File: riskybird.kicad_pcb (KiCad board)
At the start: 2 copper layers, 58.3 x 58.3 mm, 81 parts, among them J1 USB_B_Micro, J2 Conn_01x02, J3 Conn_01x02, J4 Conn_01x02, J5 Conn_01x02, J6 Conn_01x02, J7 Conn_01x10, J8 Conn_01x10, Q1 SI2302, Q2 SI2302, Q3 SI2302, Q4 SI2302, Q5 DNBT8105-7, Q6 DNBT8105-7, Q7 Q_NMOS_GSD, SW1 SW_SPST, SW2 SW_SPST, SW3 SW_SPST, U1 MCP73831-2-OT, U10 74LVC2G08, U3 TPS2113A, U4 LP2985-3.0, U6 ESP32-C3-WROOM-02, U7 BMI088, U8 FT231XS

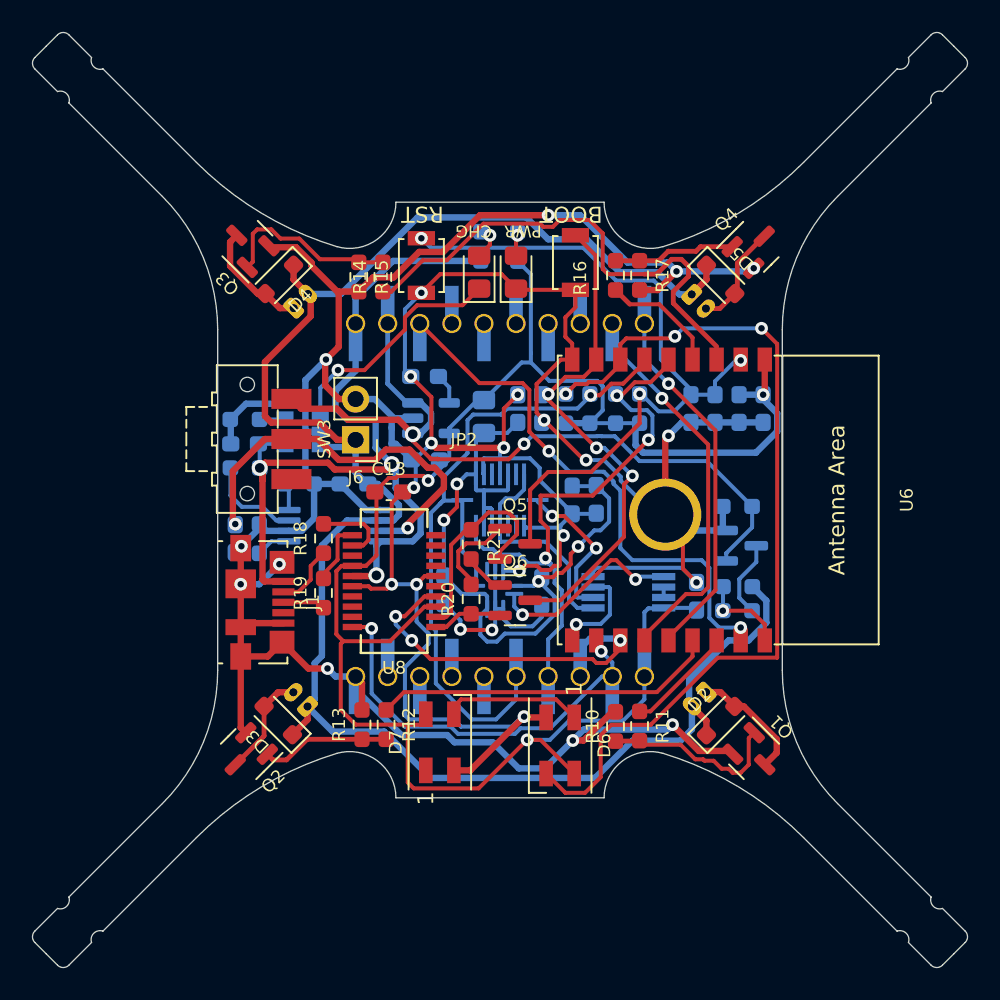
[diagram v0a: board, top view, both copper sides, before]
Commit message: finish 0.0 version
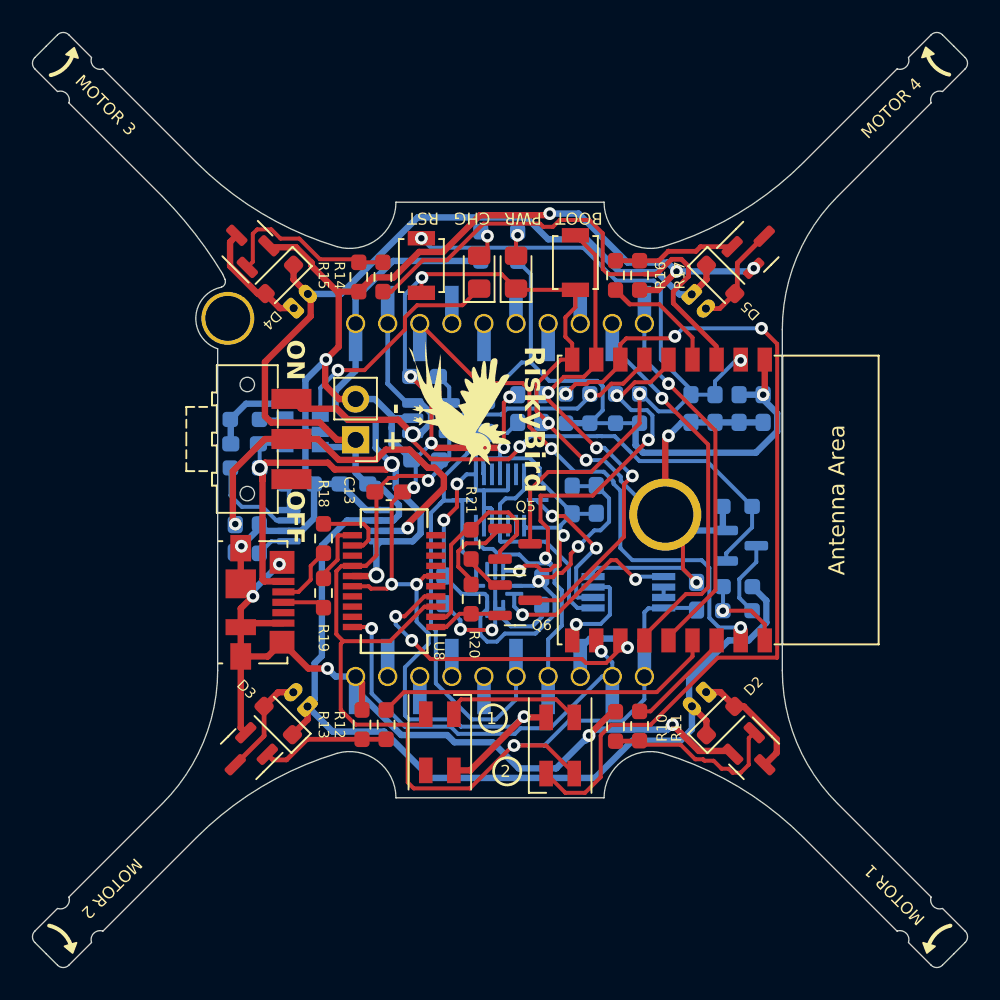
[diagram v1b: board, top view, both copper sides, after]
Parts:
- added G***: LOGO, LOGO, F.Cu at (97.4, 93.8)
- added G***: LOGO, LOGO, B.Cu at (88.6, 106.4)
- added REF**: wire_hole, riskybird:wire_hole, F.Cu at (83.0, 88.7)
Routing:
- net GNDD: track 112.3 -> 114.1 mm
- net VDD: track 112.7 -> 113.4 mm
- net /U0TXD: track 24.0 -> 24.5 mm
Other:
- outline, holes or cut-outs redrawn
- board text added: "+"
- board text added: "+5V"
- board text added: "-"
- board text added: "1"
- board text added: "2"
- board text added: "Dima Nikiforov"
- board text added: "GND"
- board text added: "MOTOR 1"
- board text added: "MOTOR 2"
- board text added: "MOTOR 3"
- board text added: "MOTOR 4"
- board text added: "OFF"
- board text added: "ON"
- board text added: "OW"
- board text added: "RX0"
- board text added: "RX1"
- board text added: "RiskyBird"
- board text added: "RiskyBird V0.0"
- board text added: "SCL"
- board text added: "SDA"
- board text added: "TX0"
- board text added: "TX1"
- board text added: "VCOM"
- board text added: "VDD"
